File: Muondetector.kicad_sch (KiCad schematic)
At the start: 32 parts, among them U2 ${SIM.PARAMS}, U3 ${SIM.PARAMS}

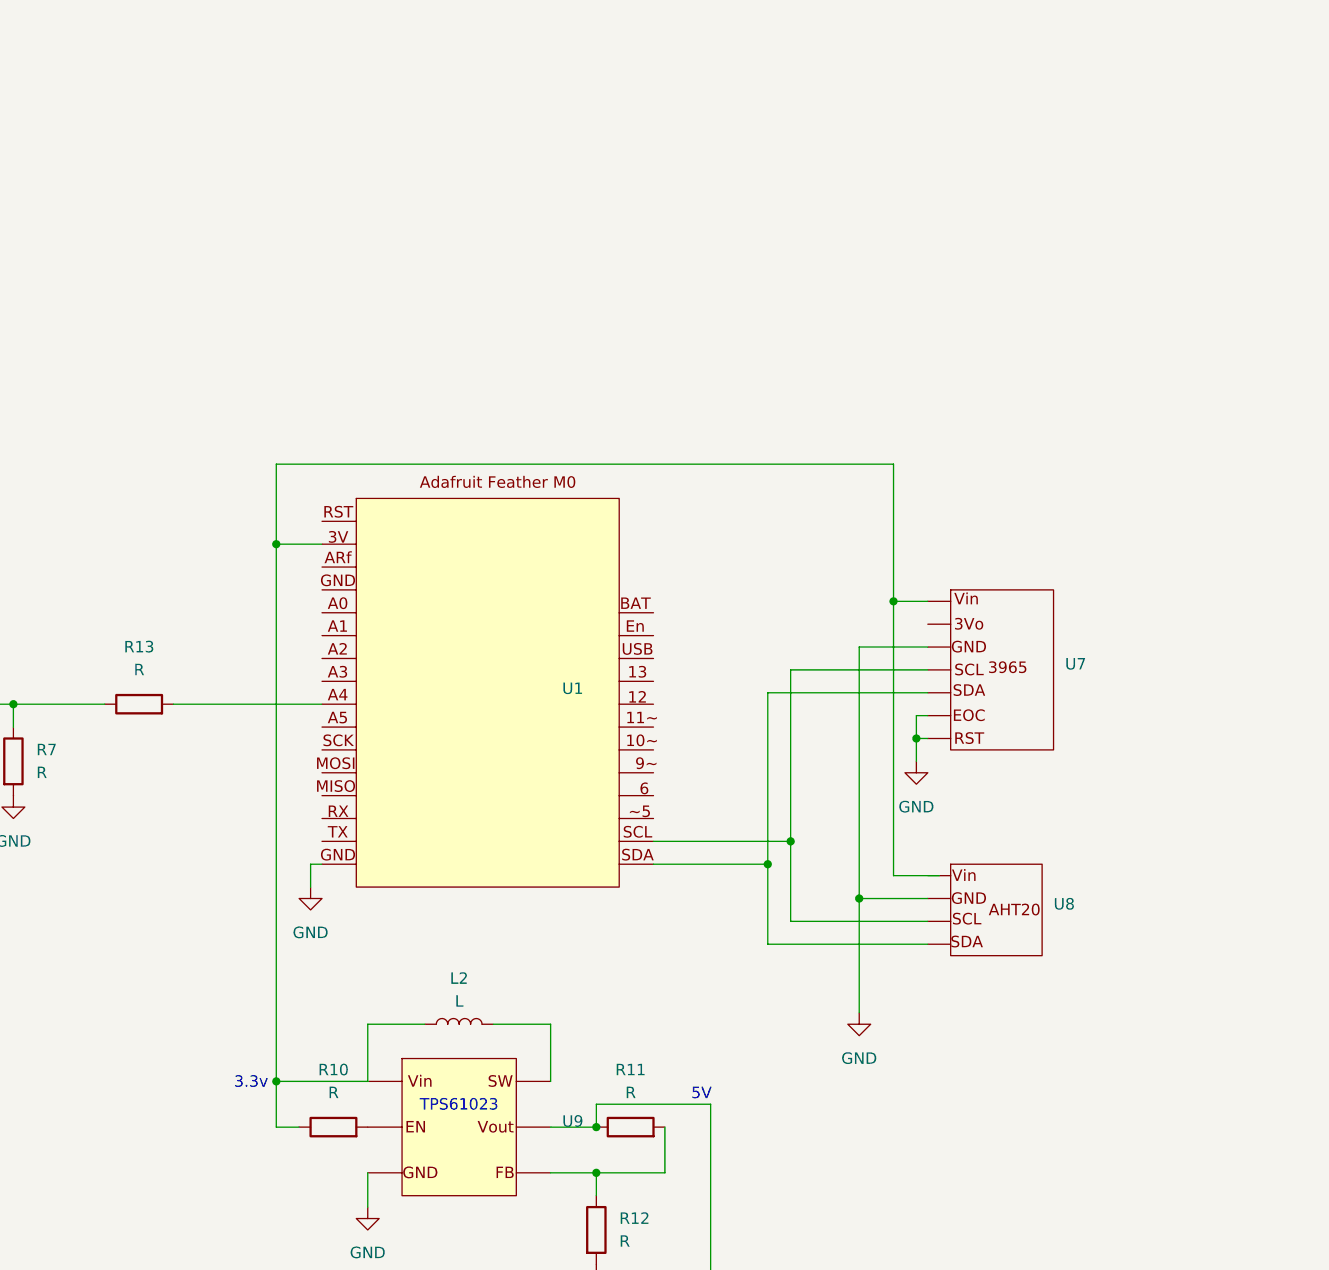
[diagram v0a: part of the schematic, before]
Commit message: yes
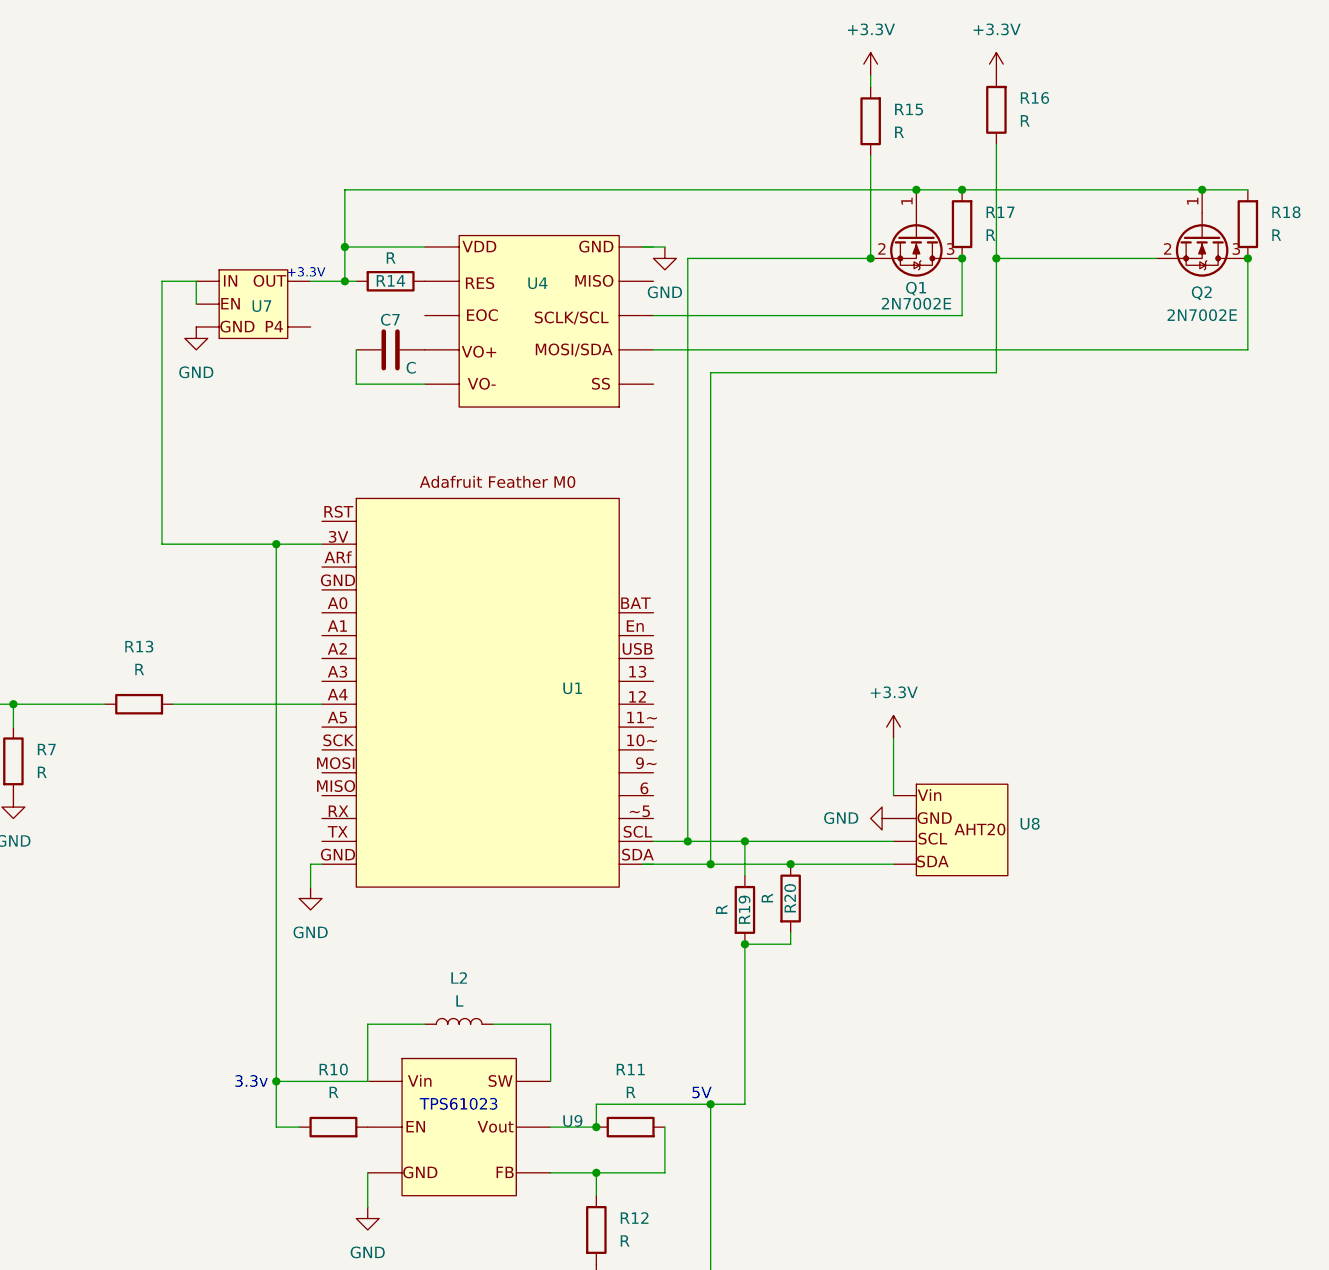
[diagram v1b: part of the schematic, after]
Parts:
- removed U7: ~, symbol MuonDetector:3965_pressure_sensor
- added C7: C, symbol Device:C
- added Q1, Q2: 2N7002E, Package_TO_SOT_SMD:SOT-23, symbol Transistor_FET:2N7002E
- added R14, R15, R16, R17, R18, R19, R20: R, symbol Device:R
- added U4: ~, symbol MuonDetector:MPR_Pressure_sensor
- added U7: ~, symbol MuonDetector:MIC5225
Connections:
- net at L1.2, R11.1, U2.3 (V+)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: now also R19.2, R20.2
- new net: Q1.2 (S), R15.1, R19.1
- new net: Q2.2 (S), R16.1, R20.1
- new net: Q1.3 (D), R17.1
- new net: Q1.1 (G), Q2.1 (G), R14.2, R17.2, R18.2
- new net: Q2.3 (D), R18.1
- new net +3.3V: R15.2, R16.2
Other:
- note added: "+3.3V"
